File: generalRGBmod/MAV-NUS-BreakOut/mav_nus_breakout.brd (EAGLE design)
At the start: 8.7 x 13.3 mm, 24 parts

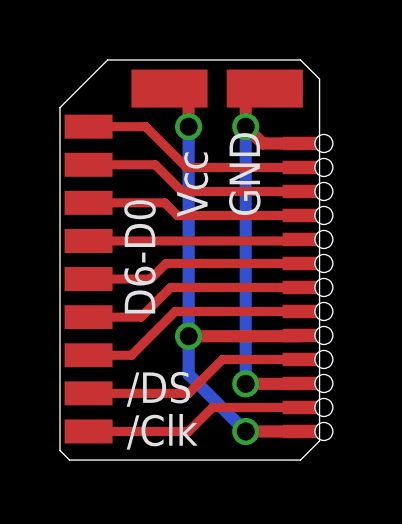
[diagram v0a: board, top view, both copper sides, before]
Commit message: initial commit DIY projects
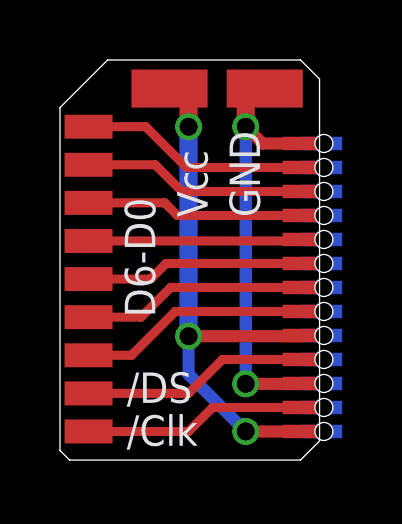
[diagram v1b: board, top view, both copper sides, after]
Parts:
- added U$23, U$24, U$25, U$26, U$27, U$28, U$29, U$30, U$31, U$32, U$33, U$34, U$35: SMD0,45, wirepad:SMD0,45-1,35
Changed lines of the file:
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@@
 <?xml version="1.0" encoding="utf-8"?>
 <!DOCTYPE eagle SYSTEM "eagle.dtd">
-<eagle version="7.6.0">
+<eagle version="7.7.0">
 <drawing>
 <settings>
@@
 <element name="U$8" library="wirepad" package="SMD0,45-1,35" value="SMD0,45" x="10.16" y="9.27" smashed="yes"/>
 <element name="U$9" library="wirepad" package="SMD0,45-1,35" value="SMD0,45" x="10.16" y="10.07" smashed="yes"/>
+<element name="U$23" library="wirepad" package="SMD0,45-1,35" value="SMD0,45" x="10.795" y="1.27" rot="MR0"/>
+<element name="U$24" library="wirepad" package="SMD0,45-1,35" value="SMD0,45" x="10.795" y="10.87" rot="MR0"/>
+<element name="U$25" library="wirepad" package="SMD0,45-1,35" value="SMD0,45" x="10.795" y="10.07" rot="MR0"/>
+<element name="U$26" library="wirepad" package="SMD0,45-1,35" value="SMD0,45" x="10.795" y="9.27" rot="MR0"/>
+<element name="U$27" library="wirepad" package="SMD0,45-1,35" value="SMD0,45" x="10.795" y="8.47" rot="MR0"/>
+<element name="U$28" library="wirepad" package="SMD0,45-1,35" value="SMD0,45" x="10.795" y="7.67" rot="MR0"/>
+<element name="U$29" library="wirepad" package="SMD0,45-1,35" value="SMD0,45" x="10.795" y="6.87" rot="MR0"/>
+<element name="U$30" library="wirepad" package="SMD0,45-1,35" value="SMD0,45" x="10.795" y="6.07" rot="MR0"/>
+<element name="U$31" library="wirepad" package="SMD0,45-1,35" value="SMD0,45" x="10.795" y="5.27" rot="MR0"/>
+<element name="U$32" library="wirepad" package="SMD0,45-1,35" value="SMD0,45" x="10.795" y="4.47" rot="MR0"/>
+<element name="U$33" library="wirepad" package="SMD0,45-1,35" value="SMD0,45" x="10.795" y="3.67" rot="MR0"/>
+<element name="U$34" library="wirepad" package="SMD0,45-1,35" value="SMD0,45" x="10.795" y="2.87" rot="MR0"/>
+<element name="U$35" library="wirepad" package="SMD0,45-1,35" value="SMD0,45" x="10.795" y="2.07" rot="MR0"/>
 </elements>
 <signals>
@@
 <wire x1="10.135" y1="4.445" x2="10.16" y2="4.47" width="0.3556" layer="1"/>
 <via x="6.35" y="11.43" extent="1-16" drill="0.6"/>
-<wire x1="6.35" y1="11.43" x2="6.35" y2="12.7" width="0.4064" layer="1"/>
+<wire x1="6.35" y1="11.43" x2="6.35" y2="12.7" width="0.6096" layer="1"/>
 <wire x1="6.35" y1="12.7" x2="5.715" y2="12.7" width="0.4064" layer="1"/>
 <wire x1="8.255" y1="1.27" x2="6.35" y2="3.175" width="0.4064" layer="16"/>
 <wire x1="6.35" y1="3.175" x2="6.35" y2="4.445" width="0.4064" layer="16"/>
-<wire x1="6.35" y1="4.445" x2="6.35" y2="11.43" width="0.4064" layer="16"/>
+<wire x1="6.35" y1="4.445" x2="6.35" y2="11.43" width="0.6096" layer="16"/>
 </signal>
 <signal name="N$11">
@@
 <wire x1="8.255" y1="2.8575" x2="10.1475" y2="2.8575" width="0.4064" layer="1"/>
 <wire x1="10.1475" y1="2.8575" x2="10.16" y2="2.87" width="0.3556" layer="1"/>
-<wire x1="8.255" y1="11.43" x2="8.255" y2="12.7" width="0.4064" layer="1"/>
+<wire x1="8.255" y1="11.43" x2="8.255" y2="12.7" width="0.6096" layer="1"/>
 <wire x1="8.255" y1="12.7" x2="8.89" y2="12.7" width="0.3556" layer="1"/>
 </signal>
